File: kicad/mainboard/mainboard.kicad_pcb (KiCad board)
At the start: 2 copper layers, 40 x 57 mm, 29 parts, among them J1 USB_C_Receptacle_USB2.0_16P, J2 Conn_01x03_Socket, J3 Conn_01x06_Socket, J4 Conn_01x06_Socket, U1 TPD1E05U06DYA, U2 TPD1E05U06DYA, U3 ESP32-S3-WROOM-1, U4 TPD1E05U06DYA, U5 TLV1117-33

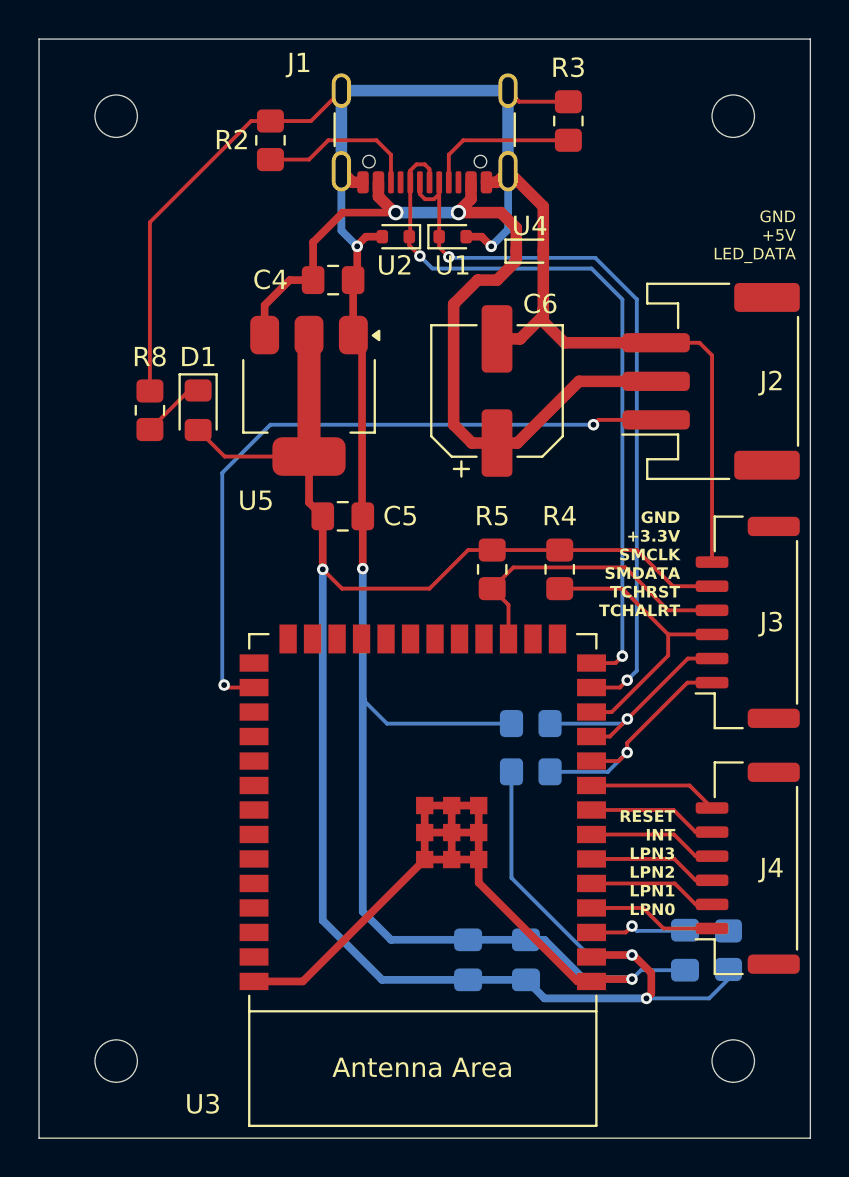
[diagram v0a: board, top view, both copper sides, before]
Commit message: change led to 11
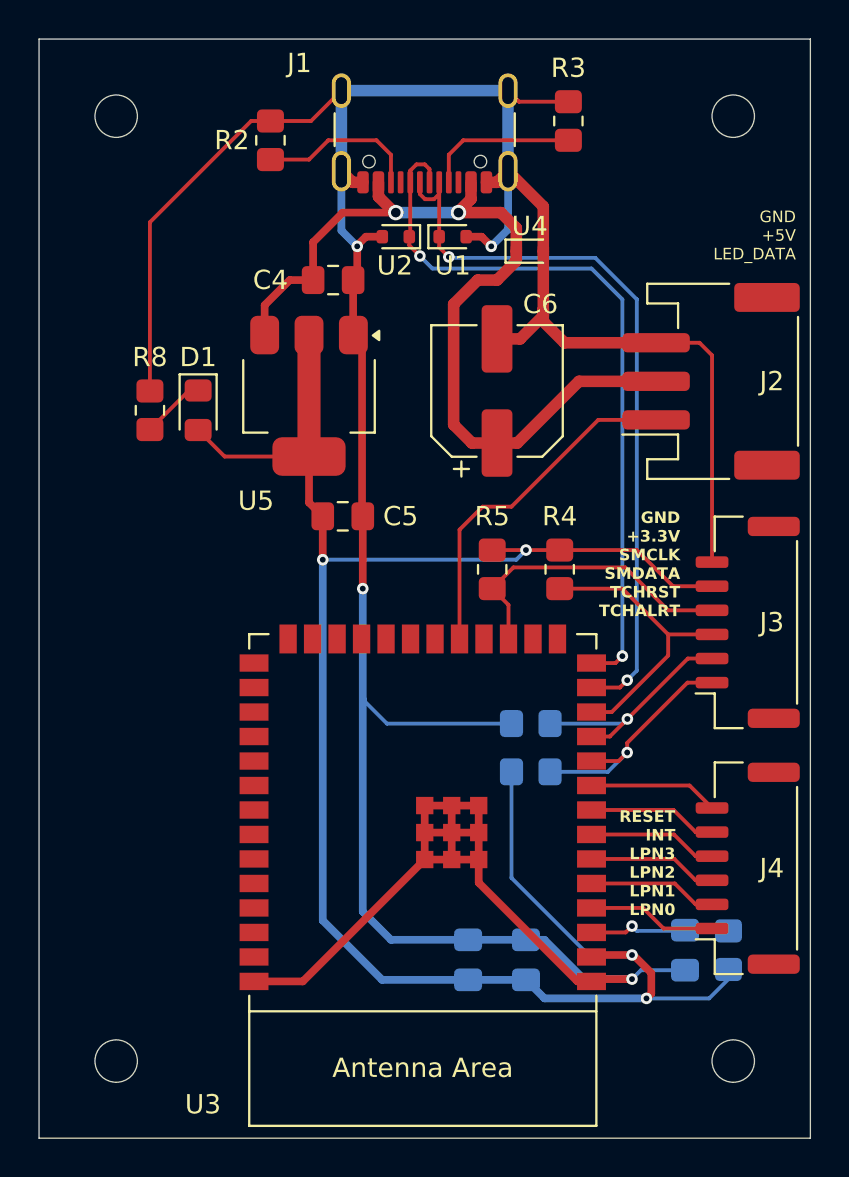
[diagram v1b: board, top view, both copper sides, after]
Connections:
- U3 pad 19: unconnected-(U3-GPIO11/TOUCH11/ADC2_CH0/FSPID/FSPIIO5/SUBSPID-Pad19) -> LED_DATA
- U3 pad 28: LED_DATA -> unconnected-(U3-SPIIO6/GPIO35/FSPID/SUBSPID-Pad28)
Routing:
- net LED_DATA: track 36.3 -> 18.2 mm, vias 2 -> 0
- net +3.3V: track 101.1 -> 101.8 mm, vias 3 -> 4
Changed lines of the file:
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@@
 	(net 36 "unconnected-(U3-GPIO1{slash}TOUCH1{slash}ADC1_CH0-Pad39)")
 	(net 37 "unconnected-(U3-GPIO14{slash}TOUCH14{slash}ADC2_CH3{slash}FSPIWP{slash}FSPIDQS{slash}SUBSPIWP-Pad22)")
-	(net 38 "unconnected-(U3-GPIO11{slash}TOUCH11{slash}ADC2_CH0{slash}FSPID{slash}FSPIIO5{slash}SUBSPID-Pad19)")
+	(net 38 "unconnected-(U3-SPIIO6{slash}GPIO35{slash}FSPID{slash}SUBSPID-Pad28)")
 	(net 39 "unconnected-(U3-GPIO12{slash}TOUCH12{slash}ADC2_CH1{slash}FSPICLK{slash}FSPIIO6{slash}SUBSPICLK-Pad20)")
 	(net 40 "unconnected-(U3-MTMS{slash}GPIO42-Pad35)")
@@
 			(size 1.5 0.9)
 			(layers "F.Cu" "F.Mask" "F.Paste")
-			(net 38 "unconnected-(U3-GPIO11{slash}TOUCH11{slash}ADC2_CH0{slash}FSPID{slash}FSPIIO5{slash}SUBSPID-Pad19)")
+			(net 34 "LED_DATA")
 			(pinfunction "GPIO11/TOUCH11/ADC2_CH0/FSPID/FSPIIO5/SUBSPID")
-			(pintype "bidirectional+no_connect")
+			(pintype "bidirectional")
 		)
 		(pad "20" smd rect
@@
 			(size 1.5 0.9)
 			(layers "F.Cu" "F.Mask" "F.Paste")
-			(net 34 "LED_DATA")
+			(net 38 "unconnected-(U3-SPIIO6{slash}GPIO35{slash}FSPID{slash}SUBSPID-Pad28)")
 			(pinfunction "SPIIO6/GPIO35/FSPID/SUBSPID")
-			(pintype "bidirectional")
+			(pintype "bidirectional+no_connect")
 		)
 		(pad "29" smd rect
@@
 	)
 	(segment
-		(start 127.05 108)
-		(end 132.17 113.12)
+		(start 121.0375 92.75)
+		(end 121.0375 89)
 		(width 0.4)
 		(layer "F.Cu")
@@
 	)
 	(segment
-		(start 121.0375 91.7125)
-		(end 121.0375 89)
+		(start 127.05 108)
+		(end 132.17 113.12)
 		(width 0.4)
 		(layer "F.Cu")
@@
 	)
 	(via
-		(at 121.0375 91.7125)
+		(at 121.0375 92.75)
 		(size 0.6)
 		(drill 0.3)
@@
 	)
 	(segment
+		(start 121.0375 92.75)
+		(end 121.0375 98.5)
+		(width 0.4)
+		(layer "B.Cu")
+		(net 1)
+	)
+	(segment
 		(start 128.57 66.925)
 		(end 128.57 71.105)
@@
 	)
 	(segment
-		(start 121.0375 91.7125)
-		(end 121.0375 98.5)
-		(width 0.4)
-		(layer "B.Cu")
-		(net 1)
-	)
-	(segment
 		(start 128.75 99.75)
 		(end 122.2875 99.75)
@@
 	)
 	(segment
-		(start 127.75 90.75)
+		(start 129.5 90.75)
 		(end 131.25 90.75)
 		(width 0.2)
@@
 	)
 	(segment
-		(start 119.9625 92.75)
-		(end 118.9625 91.75)
+		(start 127.75 90.75)
+		(end 129.5 90.75)
 		(width 0.2)
 		(layer "F.Cu")
@@
 	)
 	(segment
-		(start 118.25 88.2875)
+		(start 118.9625 91.25)
 		(end 118.9625 89)
 		(width 0.4)
@@
 	)
 	(segment
-		(start 118.9625 91.75)
+		(start 118.25 88.2875)
 		(end 118.9625 89)
 		(width 0.4)
@@
 	)
 	(segment
-		(start 126.5 90.75)
-		(end 127.75 90.75)
-		(width 0.2)
-		(layer "F.Cu")
-		(net 3)
-	)
-	(segment
 		(start 136 113.75)
 		(end 136 112.679176)
@@
 		(net 3)
 	)
-	(segment
-		(start 124.5 92.75)
-		(end 126.5 90.75)
-		(width 0.2)
-		(layer "F.Cu")
-		(net 3)
-	)
-	(segment
-		(start 119.9625 92.75)
-		(end 124.5 92.75)
-		(width 0.2)
-		(layer "F.Cu")
+	(via
+		(at 129.5 90.75)
+		(size 0.6)
+		(drill 0.3)
+		(layers "F.Cu" "B.Cu")
 		(net 3)
 	)
@@
 	)
 	(via
-		(at 118.9625 91.75)
+		(at 118.9625 91.25)
 		(size 0.6)
 		(drill 0.3)
@@
 	)
 	(segment
-		(start 118.9625 91.75)
-		(end 118.9625 109.9625)
+		(start 118.9625 109.9625)
+		(end 122.0375 113.0375)
 		(width 0.4)
 		(layer "B.Cu")
@@
 	)
 	(segment
+		(start 129.5 90.75)
+		(end 129 91.25)
+		(width 0.2)
+		(layer "B.Cu")
+		(net 3)
+	)
+	(segment
 		(start 132.75 111.75)
 		(end 135 111.75)
@@
 	)
 	(segment
-		(start 122.0375 113.0375)
-		(end 129.5 113.0375)
-		(width 0.4)
-		(layer "B.Cu")
-		(net 3)
-	)
-	(segment
 		(start 128.75 107.75)
 		(end 132.75 111.75)
@@
 	)
 	(segment
-		(start 118.9625 109.9625)
-		(end 122.0375 113.0375)
+		(start 122.0375 113.0375)
+		(end 129.5 113.0375)
+		(width 0.4)
+		(layer "B.Cu")
+		(net 3)
+	)
+	(segment
+		(start 118.9625 91.25)
+		(end 118.9625 109.9625)
 		(width 0.4)
 		(layer "B.Cu")
@@
 	)
 	(segment
+		(start 129 91.25)
+		(end 118.9625 91.25)
+		(width 0.2)
+		(layer "B.Cu")
+		(net 3)
+	)
+	(segment
 		(start 135.75 114)
 		(end 139 114)
@@
 	)
 	(segment
-		(start 113.85 97.75)
-		(end 113.98 97.88)
+		(start 128.75 88.5)
+		(end 127.25 88.5)
 		(width 0.2)
 		(layer "F.Cu")
@@
 	)
 	(segment
-		(start 113.98 97.88)
-		(end 115.4 97.88)
+		(start 127.25 88.5)
+		(end 126.055 89.695)
 		(width 0.2)
 		(layer "F.Cu")
@@
 	(segment
 		(start 133.25 84)
-		(end 133 84.25)
+		(end 128.75 88.5)
 		(width 0.2)
 		(layer "F.Cu")
 		(net 34)
 	)
-	(via
-		(at 113.85 97.75)
-		(size 0.6)
-		(drill 0.3)
-		(layers "F.Cu" "B.Cu")
-		(net 34)
-	)
-	(via
-		(at 133 84.25)
-		(size 0.6)
-		(drill 0.3)
-		(layers "F.Cu" "B.Cu")
-		(net 34)
-	)
-	(segment
-		(start 116.25 84.25)
-		(end 133 84.25)
-		(width 0.2)
-		(layer "B.Cu")
-		(net 34)
-	)
 	(segment
-		(start 113.85 97.75)
-		(end 113.75 97.65)
+		(start 126.055 89.695)
+		(end 126.055 95.36)
 		(width 0.2)
-		(layer "B.Cu")
-		(net 34)
-	)
-	(segment
-		(start 113.75 97.65)
-		(end 113.75 86.75)
-		(width 0.2)
-		(layer "B.Cu")
-		(net 34)
-	)
-	(segment
-		(start 113.75 86.75)
-		(end 116.25 84.25)
-		(width 0.2)
-		(layer "B.Cu")
+		(layer "F.Cu")
 		(net 34)
 	)

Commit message: final tweaks
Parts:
- moved G*** 2.02 mm to (109.5, 110.0)
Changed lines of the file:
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@@
 	(footprint "Logo:Snep_Copper"
 		(layer "F.Cu")
-		(at 109.25 108)
+		(at 109.5 110)
 		(property "Reference" "G***"
 			(at 0 0 0)
